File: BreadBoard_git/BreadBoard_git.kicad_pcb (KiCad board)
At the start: 4 copper layers, 119 x 62.6 mm, 88 parts, among them J1 PD-40, J2 USB_C_Receptacle_USB2.0_14P, J4 Conn_01x02_Pin, J5 Conn_01x02_Pin, J7 Conn_01x15_Pin, J8 Conn_01x05_Pin, Q1 CSD18512Q5B, Q3 CSD18512Q5B, Q5 RQ3E110AJTB, Q6 RQ3E110AJTB, SW1 SKRPADE010, SW2 SKRPADE010, U2 LM61460AANRJRR, U3 LM5148RGYR, U4 AMS1117-3.3, U5 ESP32-S3-WROOM-1

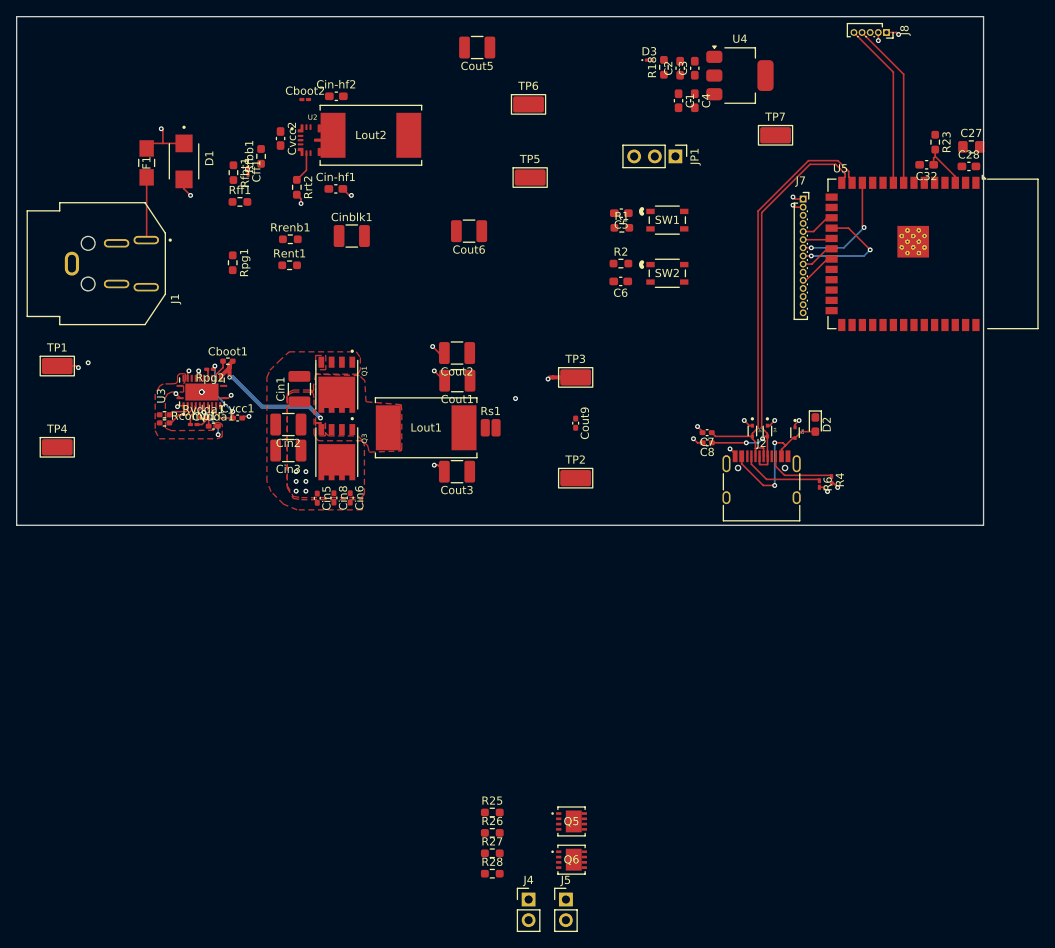
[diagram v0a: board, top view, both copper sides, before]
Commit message: updates!
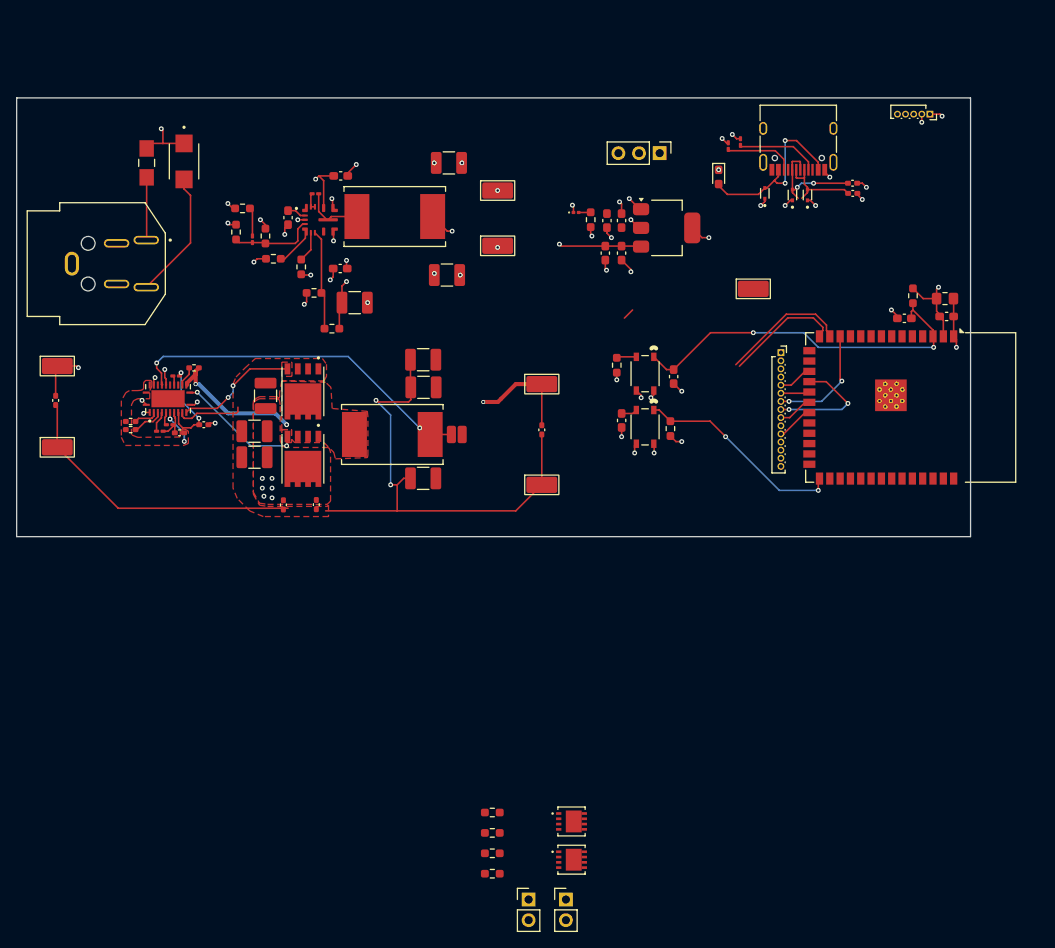
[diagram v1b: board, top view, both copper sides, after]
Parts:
- moved J2 43.6 mm to (170.4, 53.6), turned to 180 degrees
- moved R6 43.2 mm to (163.3, 54.2), turned to 90 degrees
- moved R4 43.0 mm to (161.8, 54.7), turned to 90 degrees
- moved C8 36.6 mm to (177.1, 59.3), turned to 0 degrees
- moved Cin8 36.3 mm to (79.0, 86.0)
- moved C7 34.5 mm to (177.1, 60.5), turned to 0 degrees
- moved D2 32.7 mm to (160.6, 58.5)
- moved D5 29.8 mm to (171.5, 60.8), turned to 90 degrees
- moved D6 29.7 mm to (166.3, 60.5), turned to 90 degrees
- moved D4 29.2 mm to (169.7, 60.8), turned to 90 degrees
- moved R2 21.2 mm to (154.7, 89.5), turned to 90 degrees
- moved C5 21.1 mm to (155.1, 83.1), turned to -90 degrees
- moved R18 20.8 mm to (144.8, 63.8)
- moved C2 20.8 mm to (146.8, 63.9)
- moved U4 20.8 mm to (154.2, 64.8)
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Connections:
- Cout1 pad 2: GND -> PGND
- Cout2 pad 2: GND -> PGND
- Cout3 pad 2: GND -> PGND
- Cout9 pad 2: GND -> PGND
- D1 pad A: GND -> PGND
- J1 pad 2: GND -> PGND
- J1 pad 3: GND -> PGND
- J1 pad S1: GND -> PGND
- SW1 pad 2: unconnected-(SW1-Pad2) -> /CHIP_PU
- SW1 pad 4: unconnected-(SW1-Pad4) -> GND
- SW2 pad 2: unconnected-(SW2-Pad2) -> /BOOT
- SW2 pad 4: unconnected-(SW2-Pad4) -> GND
- TP4 pad 1: GND -> PGND
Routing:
- net PGND: track 0.10 -> 121.8 mm, vias 0 -> 2
- net /ISNS_P: track 0.00 -> 43.7 mm, vias 0 -> 2
- net /CHIP_PU: track 6.22 -> 47.8 mm, vias 0 -> 2
- net /BOOT: track 0.00 -> 27.8 mm, vias 0 -> 2
- net /USB_D-: track 54.2 -> 27.5 mm
- net /USB_D+: track 55.0 -> 28.5 mm
- net GND: track 25.4 -> 50.2 mm, vias 20 -> 40
- net /SDA: track 20.6 -> 0.03 mm
- net /SCL: track 20.5 -> 0.03 mm
- net +24V: track 13.0 -> 30.6 mm, vias 11 -> 13
- net +3.3V: track 2.96 -> 19.5 mm, vias 2 -> 7
- net /HO: track 0.00 -> 15.9 mm, vias 0 -> 2
- net /LO: track 0.00 -> 15.2 mm, vias 0 -> 2
- net Net-(U2-EN/SYNC): track 0.00 -> 12.3 mm
- net +5V: track 0.00 -> 11.6 mm, vias 0 -> 1
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- added copper zone on In2.Cu, net +5V
- added copper zone on In2.Cu, net +5V_IN
- added copper zone on In2.Cu, net +5V_USB
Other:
- board size 119 x 62.6 mm -> 117.4 x 54 mm
